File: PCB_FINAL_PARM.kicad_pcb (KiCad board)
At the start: 2 copper layers, 87.6 x 95.2 mm, 51 parts, among them J1 Conn_01x02_Servo1, J10 Conn_01x04_TRIS, J11 Conn_01x04_3v3, J2 Conn_01x03_UART1, J3 Conn_01x03_UART2, J4 Conn_01x04_PWM, J5 Conn_01x05_PROGRAMER, J6 Conn_01x02_POWER, J7 Conn_01x02_Servo2, J8 Conn_01x02_Servo3, J9 Conn_01x02_Servo4, U1 L7805, U2 DSPIC33EP128GM604, U3 LM317T/SERVO, U4 LM317T/SERVO, U5 LM317T/SERVO, U6 LM317T/SERVO, U7 AZ1117-3.3, Y1 7.3728Mhz

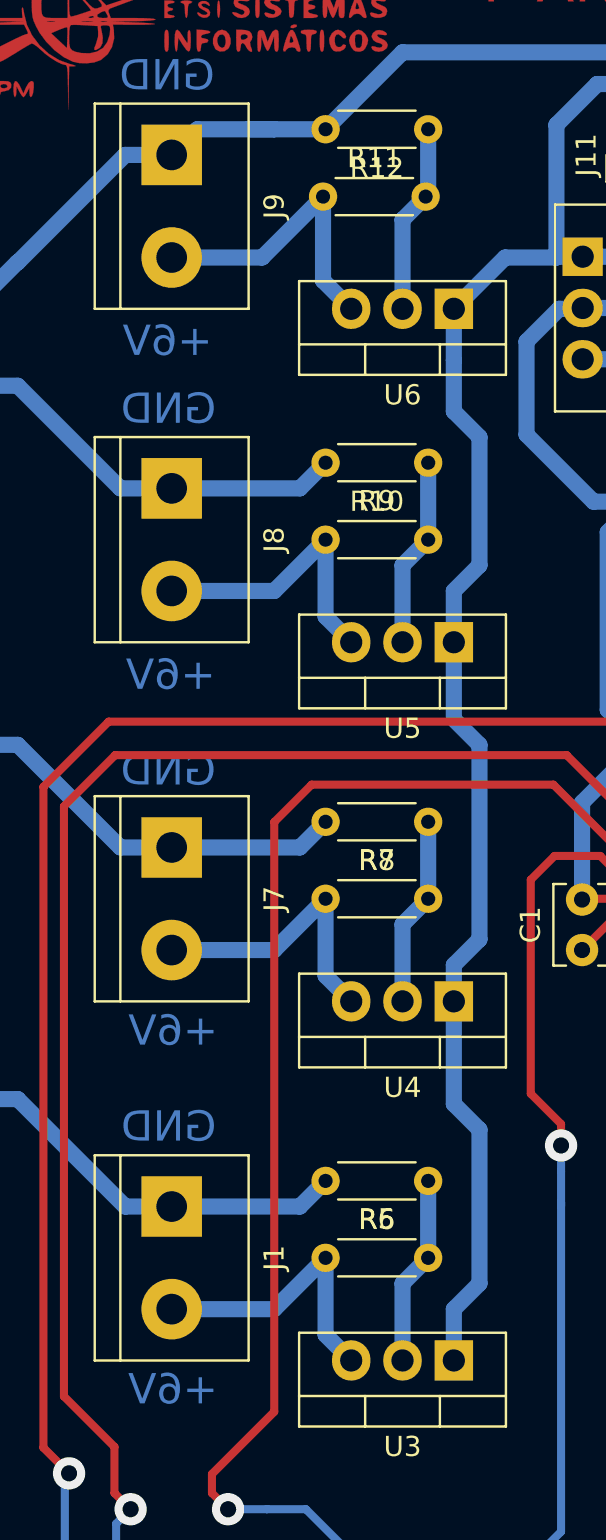
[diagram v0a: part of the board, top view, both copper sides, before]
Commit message: Arreglados los LM317
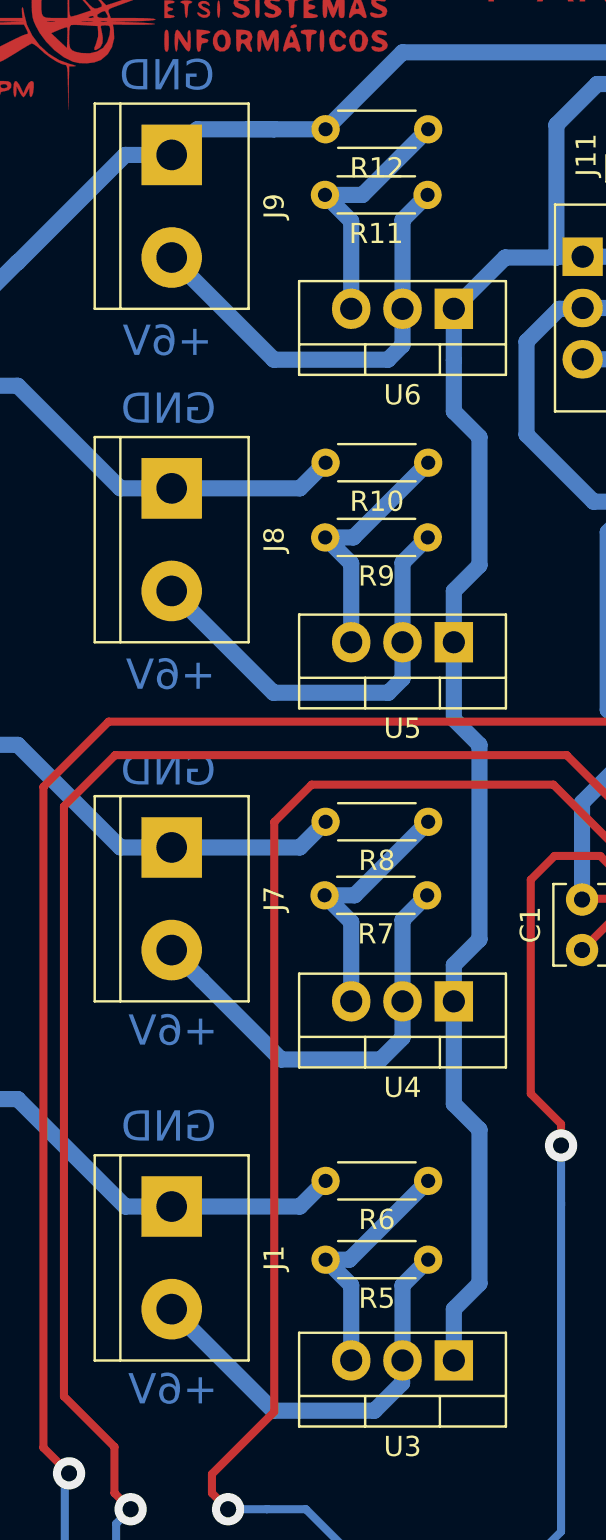
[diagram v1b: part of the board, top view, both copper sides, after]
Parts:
- moved R11 5.18 mm to (165.1, 71.8), turned to 180 degrees
- moved R5 5.08 mm to (165.1, 124.5), turned to 180 degrees
- moved R9 5.06 mm to (165.1, 88.8), turned to 180 degrees
- moved R7 5.03 mm to (165.1, 106.5), turned to 180 degrees
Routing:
- net Net-(J7-Pad2): track 14.3 -> 21.7 mm
- net Net-(J8-Pad2): track 14.3 -> 21.3 mm
- net Net-(J9-Pad2): track 14.9 -> 21.8 mm
- net Net-(J1-Pad2): track 14.3 -> 20.7 mm
- net Net-(R11-Pad2): track 9.42 -> 12.6 mm
- net Net-(R7-Pad2): track 9.42 -> 12.4 mm
- net Net-(R10-Pad1): track 9.42 -> 12.4 mm
- net Net-(R5-Pad2): track 9.42 -> 12.2 mm
